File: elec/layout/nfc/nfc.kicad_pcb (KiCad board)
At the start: 2 copper layers, 27 parts, among them U1 _NXP_Semicon_PN5321A3HN_C106_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

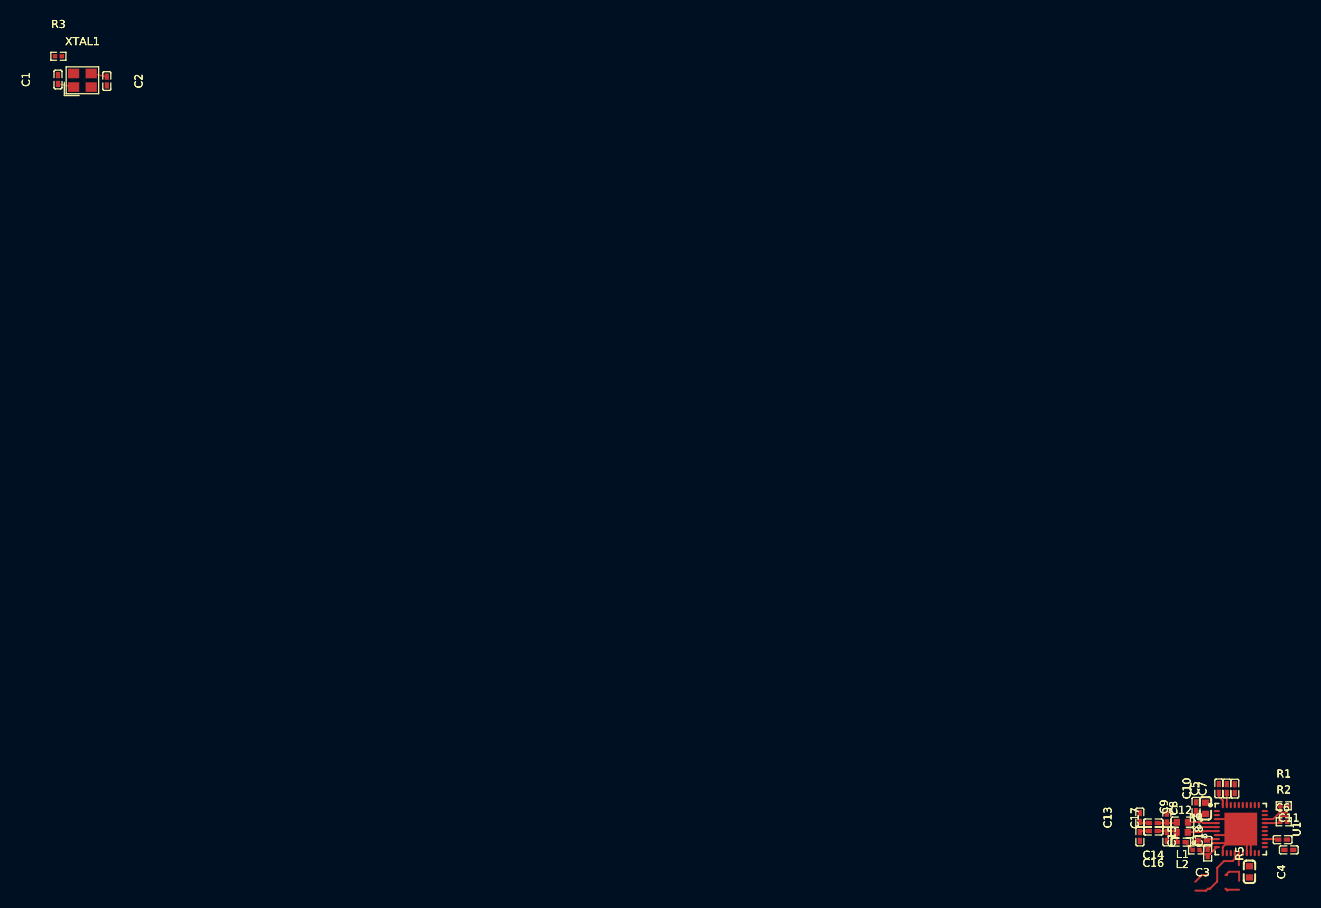
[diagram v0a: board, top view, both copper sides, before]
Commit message: Build full
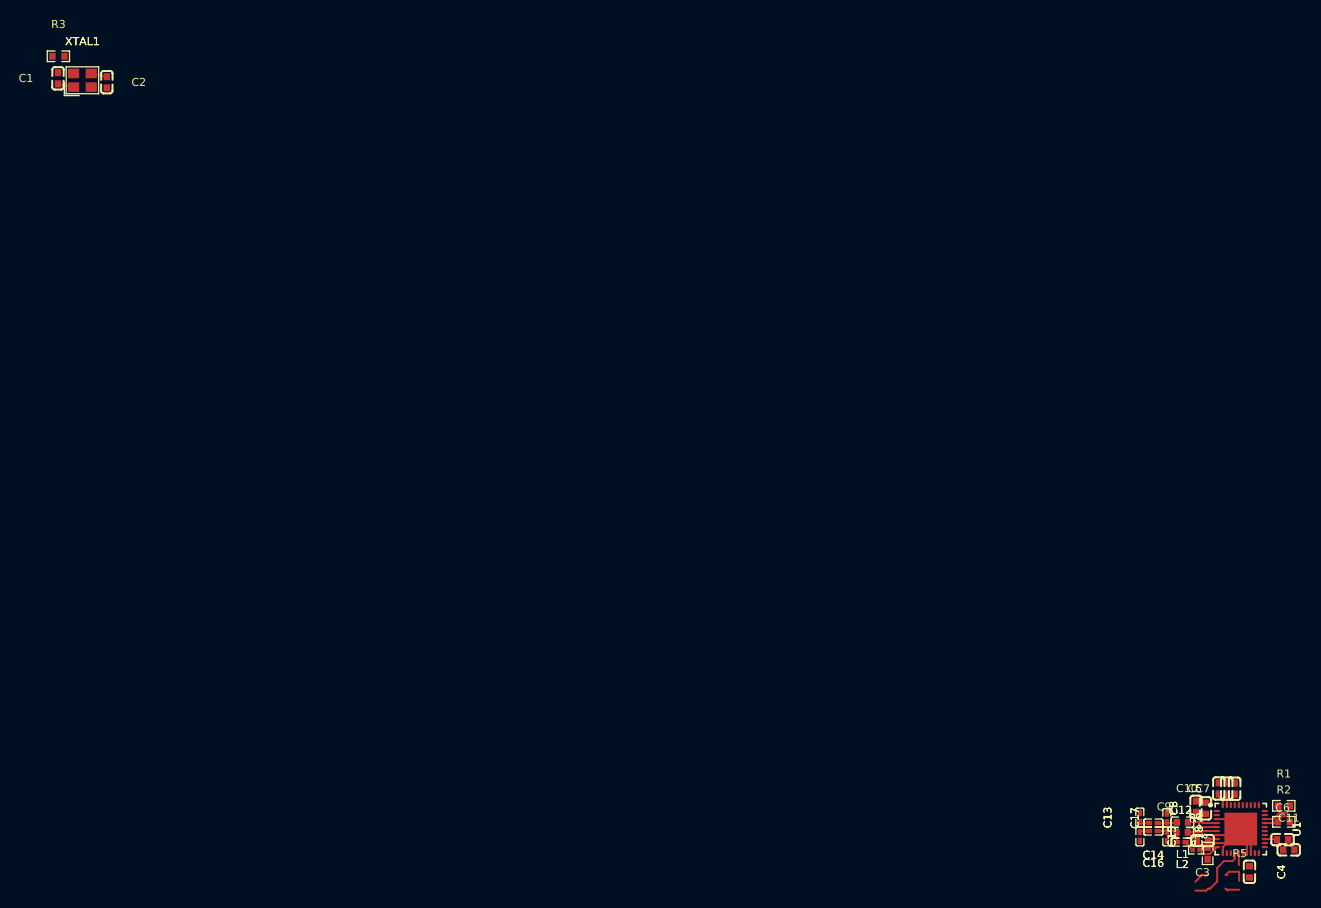
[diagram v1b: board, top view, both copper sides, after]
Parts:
- C1, C2: value 20pF ±5% 50V C0G -> 100nF ±10% 50V X7R; footprint lcsc:C0402 -> lcsc:C0603
- C10, C11, C3, C5, C6, C7, C9: value 100nF ±10% 16V X7R -> 100nF ±10% 50V X7R; footprint lcsc:C0402 -> lcsc:C0603
- C4, C8: value 10µF ±10% 10V X5R -> 100nF ±10% 50V X7R
- L1, L2: value 560nH ±5% 450mA 480mΩ -> 560nH ±5% infHz 450mA 480mΩ
- R1, R2, R3, R5: value 5.1kΩ ±1% 62.5mW -> 1kΩ ±1% 100mW; footprint lcsc:R0402 -> lcsc:R0603
- moved C1 0.15 mm to (-3.05, -0.25)
- moved C2 0.15 mm to (3.05, 0.25)
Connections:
- net power_vmid-lv renamed lv
- C10 pad 1: net-6 -> net
- C12 pad 2: net-3 -> net-13
- C13 pad 1: net -> net-11
- C14 pad 2: net -> net-11
- C15 pad 1: net-12 -> net-6
- C16 pad 2: net-12 -> net-6
- C2 pad 1: net-9 -> net-5
- C3 pad 1: net-6 -> net
- C4 pad 1: net-6 -> net
- C5 pad 1: net-6 -> net
- C6 pad 1: net-6 -> net
- C7 pad 1: net-5 -> net-2
- C7 pad 2: power_svdd-lv -> net-1
- C8 pad 1: net-6 -> net
- C9 pad 1: net-6 -> net
- L1 pad 2: net-2 -> net-10
- L2 pad 2: net-8 -> net-9
- R1 pad 1: net-10 -> net-7
- R1 pad 2: hv -> net-12
- R2 pad 1: net-7 -> net-8
- R2 pad 2: hv -> net-12
- R3 pad 2: net-11 -> net-4
- R4 pad 1: net-3 -> net-13
- R4 pad 2: net-4 -> net-3
- R5 pad 2: net-4 -> net-3
- U1 pad 10: net-4 -> net-3
- U1 pad 14: net-9 -> net-5
- U1 pad 15: net-11 -> net-4
- U1 pad 16: net-6 -> net
- U1 pad 20: nfc_ic-net -> nfc_ic.footprint.pins[12].net-net
- U1 pad 21: nfc_ic-net -> nfc_ic.footprint.pins[13].net-net
- U1 pad 22: nfc_ic-net -> nfc_ic.footprint.pins[14].net-net
- U1 pad 23: net-6 -> net
- U1 pad 25: p70_irq -> signal
- U1 pad 26: signal -> signal-1
- U1 pad 27: net-7 -> net-8
- U1 pad 28: net-10 -> net-7
- U1 pad 37: net-5 -> net-2
- U1 pad 39: net-6 -> net
- U1 pad 4: net-2 -> net-10
- U1 pad 40: net-6 -> net
- U1 pad 5: net-6 -> net
- U1 pad 6: net-8 -> net-9
- U1 pad 8: net-6 -> net
- XTAL1 pad 3: net-9 -> net-5
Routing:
- net net-5: track 1.49 -> 3.48 mm
- net net-9: track 5.90 -> 3.91 mm
